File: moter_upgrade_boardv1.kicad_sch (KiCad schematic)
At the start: 52 parts, among them J1 Conn_01x04_Socket, J2 Conn_01x03_Socket, J3 Conn_01x02_Socket, J4 Conn_01x03_Socket, J5 Conn_01x05_Socket, J6 USB_C_Receptacle_USB2.0_16P, J7 Conn_01x03_Socket, SW1 SW_SPDT, SW2 SW_Push, SW3 SW_Wuerth_450301014042, U1 BD33FC0FP, U2 TLP785, U3 TLP785, U4 STM32H523CCTx, U5 MCP2562-E-P, U6 CH340E, U7 BD33FC0FP

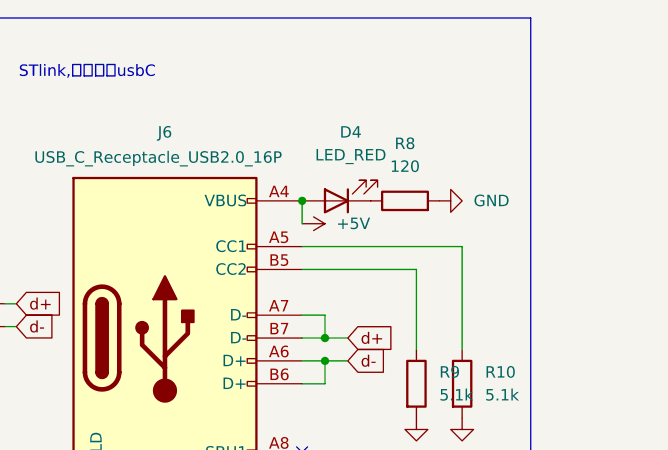
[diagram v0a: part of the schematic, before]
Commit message: usbCをもとに戻した　最終？？版
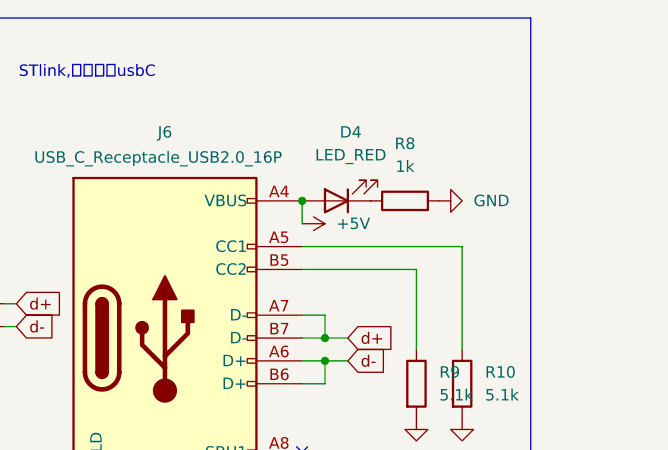
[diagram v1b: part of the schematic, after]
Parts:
- R8: value 120 -> 1k
